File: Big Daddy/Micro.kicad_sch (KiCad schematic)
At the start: 24 parts, among them Q1 2N7002, U1 MAX33054EASA+T, U2 ESP32-S3-DevKitC, U3 ESP32-S3-DevKitC

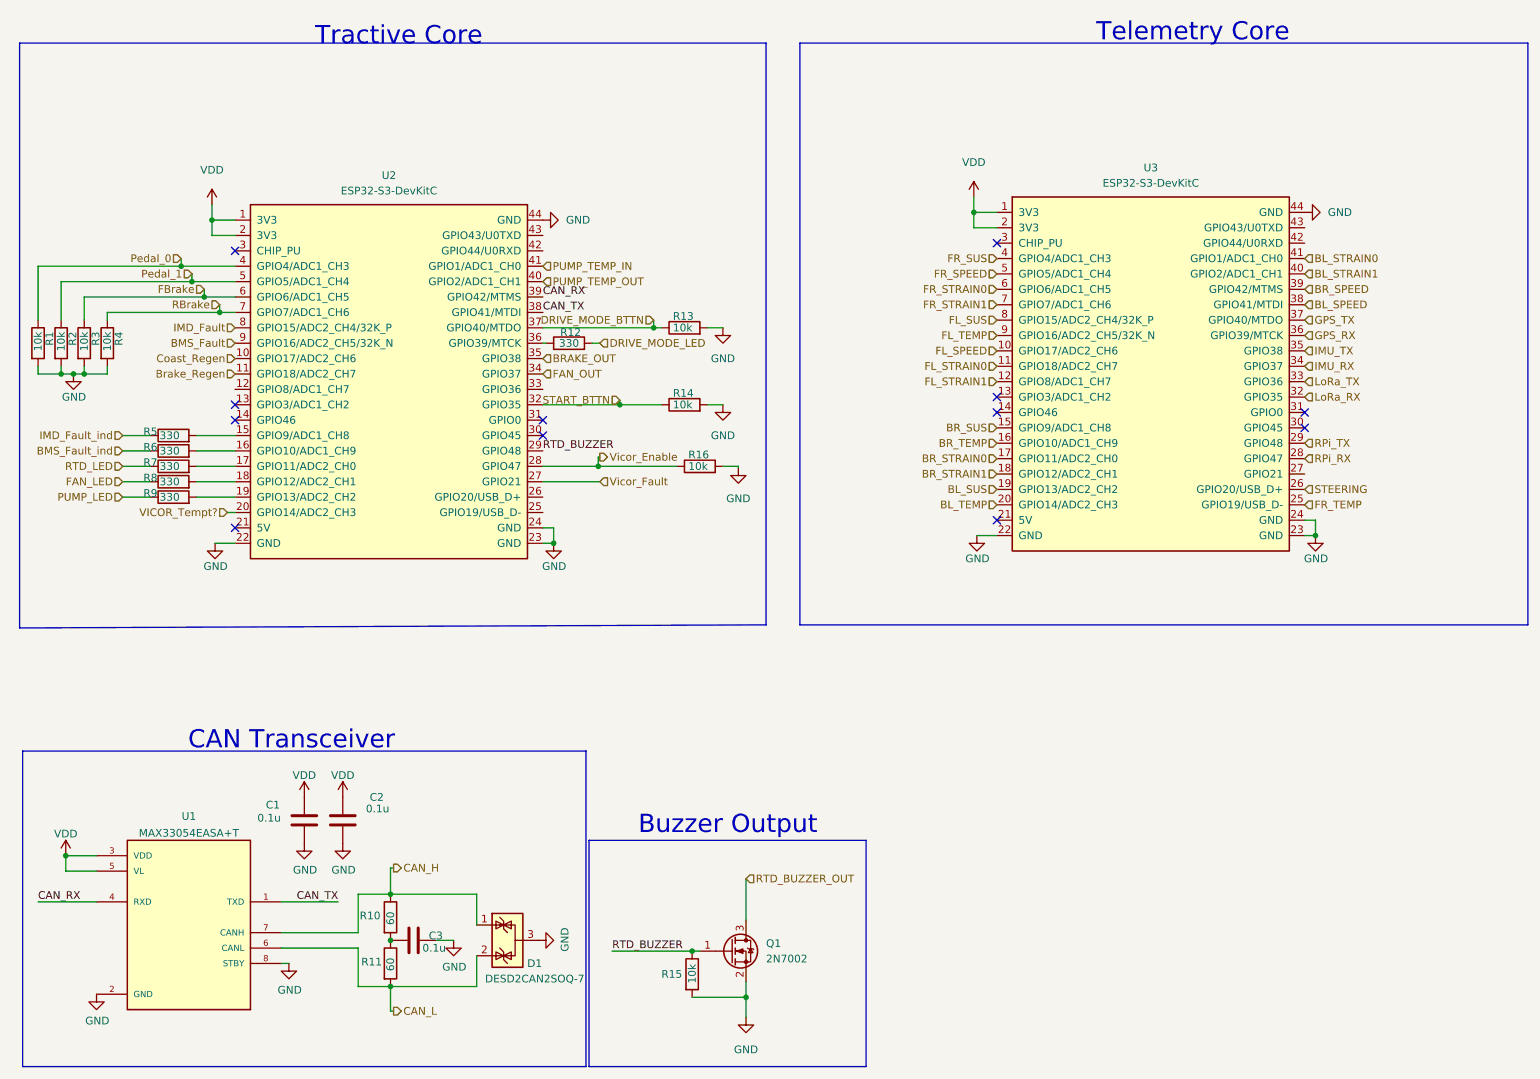
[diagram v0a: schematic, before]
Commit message: so cloes
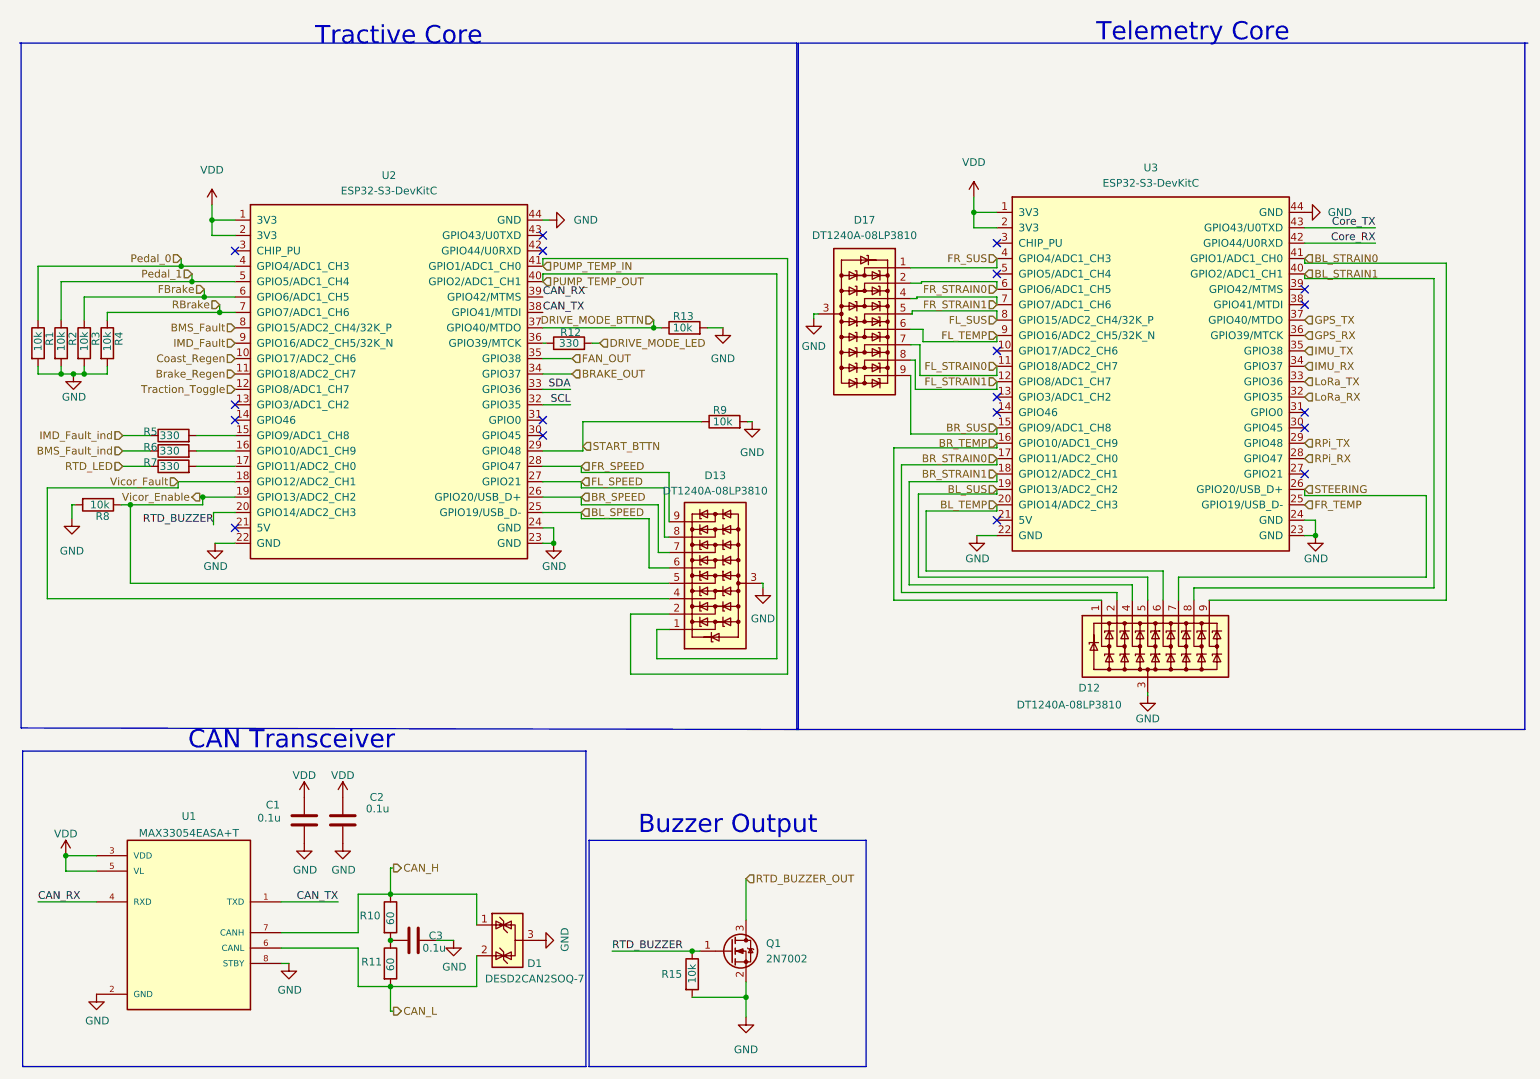
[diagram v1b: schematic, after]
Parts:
- removed R14, R16: 10k, Resistor_SMD:R_0603_1608Metric_Pad0.98x0.95mm_HandSolder, symbol Device:R
- added D12, D13, D17: DT1240A-08LP3810, Package_DFN_QFN:UDFN-9_1.0x3.8mm_P0.5mm, symbol Power_Protection:DT1240A-08LP3810
- R8, R9: value 330 -> 10k
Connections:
- net FAN_LED is gone; now on net Vicor_Enable: R8.1
- net PUMP_LED is gone; now on net START_BTTN: R9.1
- net VICOR_Tempt? is gone; now on net RTD_BUZZER: U2.20 (GPIO14/ADC2_CH3)
- net BL_SPEED: now also U2.25 (GPIO19/USB_D-), D13.6 (K5); no longer U3.38 (GPIO41/MTDI)
- net BL_STRAIN0: now also D12.9 (K8)
- net BL_STRAIN1: now also D12.8 (K7)
- net BL_SUS: now also D12.5 (K4)
- net BL_TEMP: now also D12.6 (K5)
- net BMS_Fault: now also U2.8 (GPIO15/ADC2_CH4/32K_P); no longer U2.9 (GPIO16/ADC2_CH5/32K_N)
- net BRAKE_OUT: now also U2.34 (GPIO37); no longer U2.35 (GPIO38)
- net BR_SPEED: now also U2.26 (GPIO20/USB_D+), D13.7 (K6); no longer U3.39 (GPIO42/MTMS)
- net BR_STRAIN0: now also D12.2 (K2)
- net BR_STRAIN1: now also D12.4 (K3)
- net BR_SUS: now also D17.9 (K8)
- net BR_TEMP: now also D12.1 (K1)
- net FAN_OUT: now also U2.35 (GPIO38); no longer U2.34 (GPIO37)
- net FL_SPEED: now also U2.27 (GPIO21), D13.8 (K7); no longer U3.10 (GPIO17/ADC2_CH6)
- net FL_STRAIN0: now also D17.7 (K6)
- net FL_STRAIN1: now also D17.8 (K7)
- net FL_SUS: now also D17.5 (K4)
- net FL_TEMP: now also D17.6 (K5)
- net FR_SPEED: now also U2.28 (GPIO47), D13.9 (K8); no longer U3.5 (GPIO5/ADC1_CH4)
- net FR_STRAIN0: now also D17.2 (K2)
- net FR_STRAIN1: now also D17.4 (K3)
- net FR_SUS: now also D17.1 (K1)
- net GND: now also R8.2, R9.2, D12.3 (A), D13.3 (A), D17.3 (A)
- net IMD_Fault: now also U2.9 (GPIO16/ADC2_CH5/32K_N); no longer U2.8 (GPIO15/ADC2_CH4/32K_P)
- net PUMP_TEMP_IN: now also D13.2 (K2)
- net PUMP_TEMP_OUT: now also D13.1 (K1)
- net RTD_BUZZER: no longer U2.29 (GPIO48)
- net START_BTTN: now also U2.29 (GPIO48); no longer U2.32 (GPIO35)
- net STEERING: now also D12.7 (K6)
- net Vicor_Enable: now also U2.19 (GPIO13/ADC2_CH2), D13.5 (K4); no longer U2.28 (GPIO47)
- net Vicor_Fault: now also U2.18 (GPIO12/ADC2_CH1), D13.4 (K3); no longer U2.27 (GPIO21)
- net Traction_Toggle: now reaches U2.12 (GPIO8/ADC1_CH7)
- net SDA: now reaches U2.33 (GPIO36)
- net Core_RX: now reaches U3.42 (GPIO44/U0RXD)
- net Core_TX: now reaches U3.43 (GPIO43/U0TXD)
- new net SCL: U2.32 (GPIO35)
- no-connect marks 12 -> 19
